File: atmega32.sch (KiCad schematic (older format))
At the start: 38 parts, among them J1 USB_B_Micro, J2 20021111-00016T4LF, SW1 SW_MEC_5E, U1 ATmega328P-AU, U2 FT232RL, Y1 Crystal

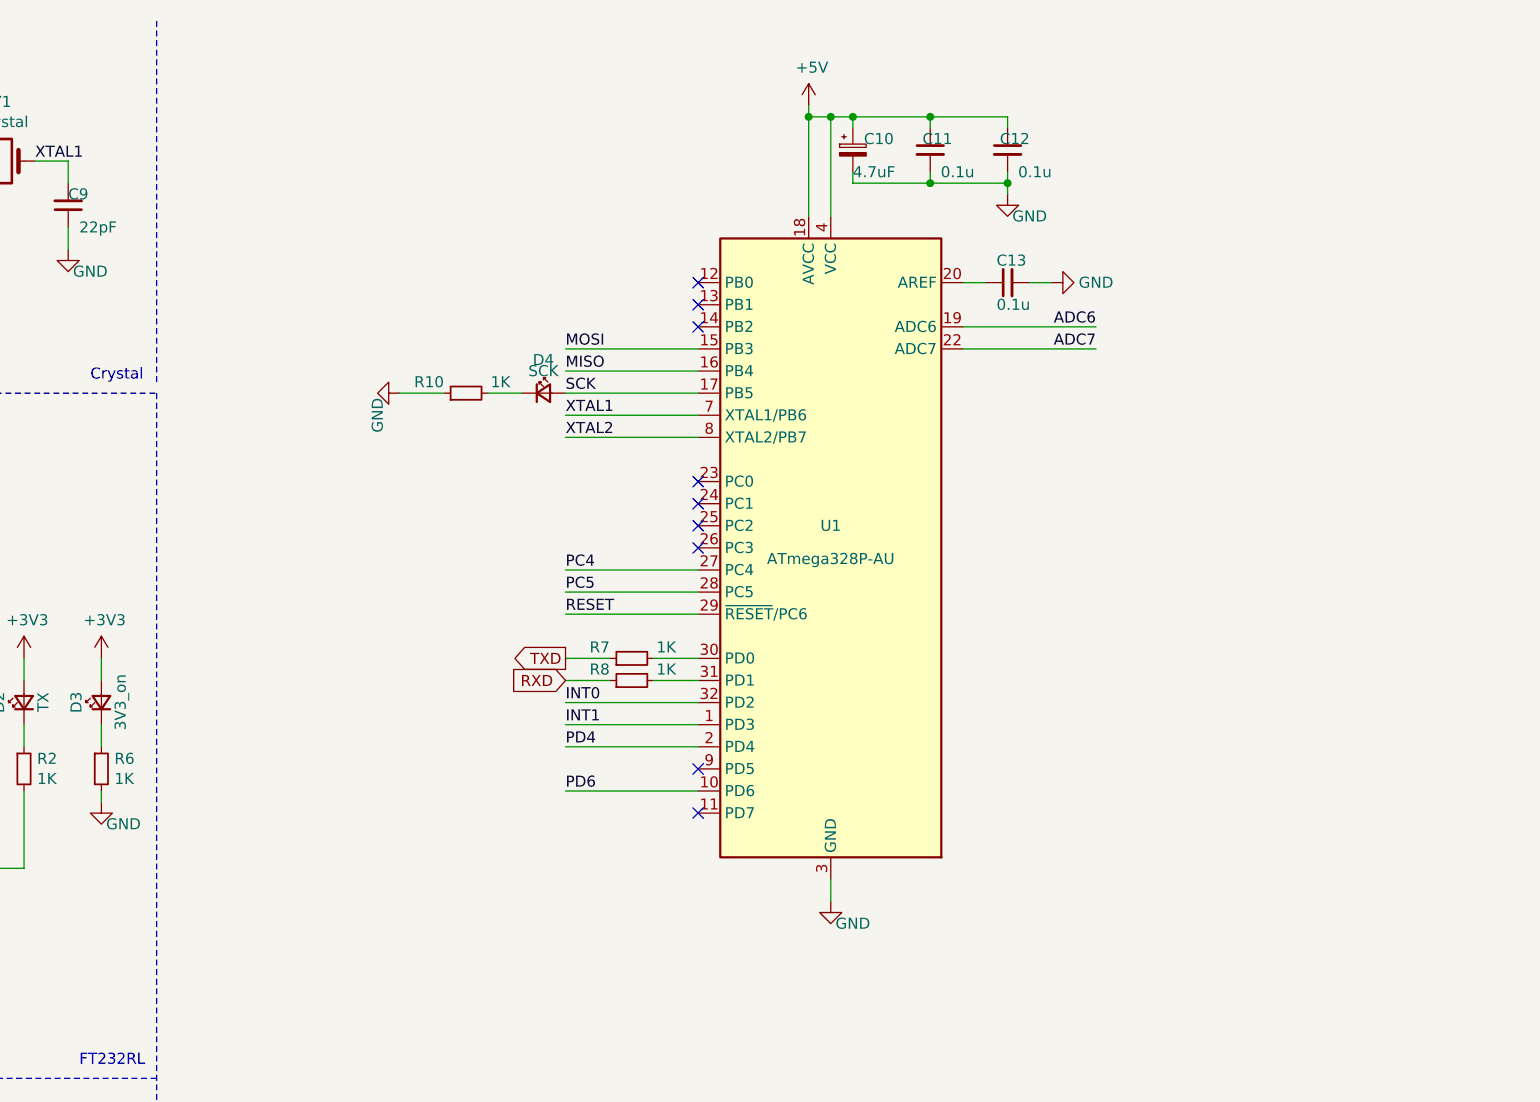
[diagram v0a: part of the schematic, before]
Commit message: orderd
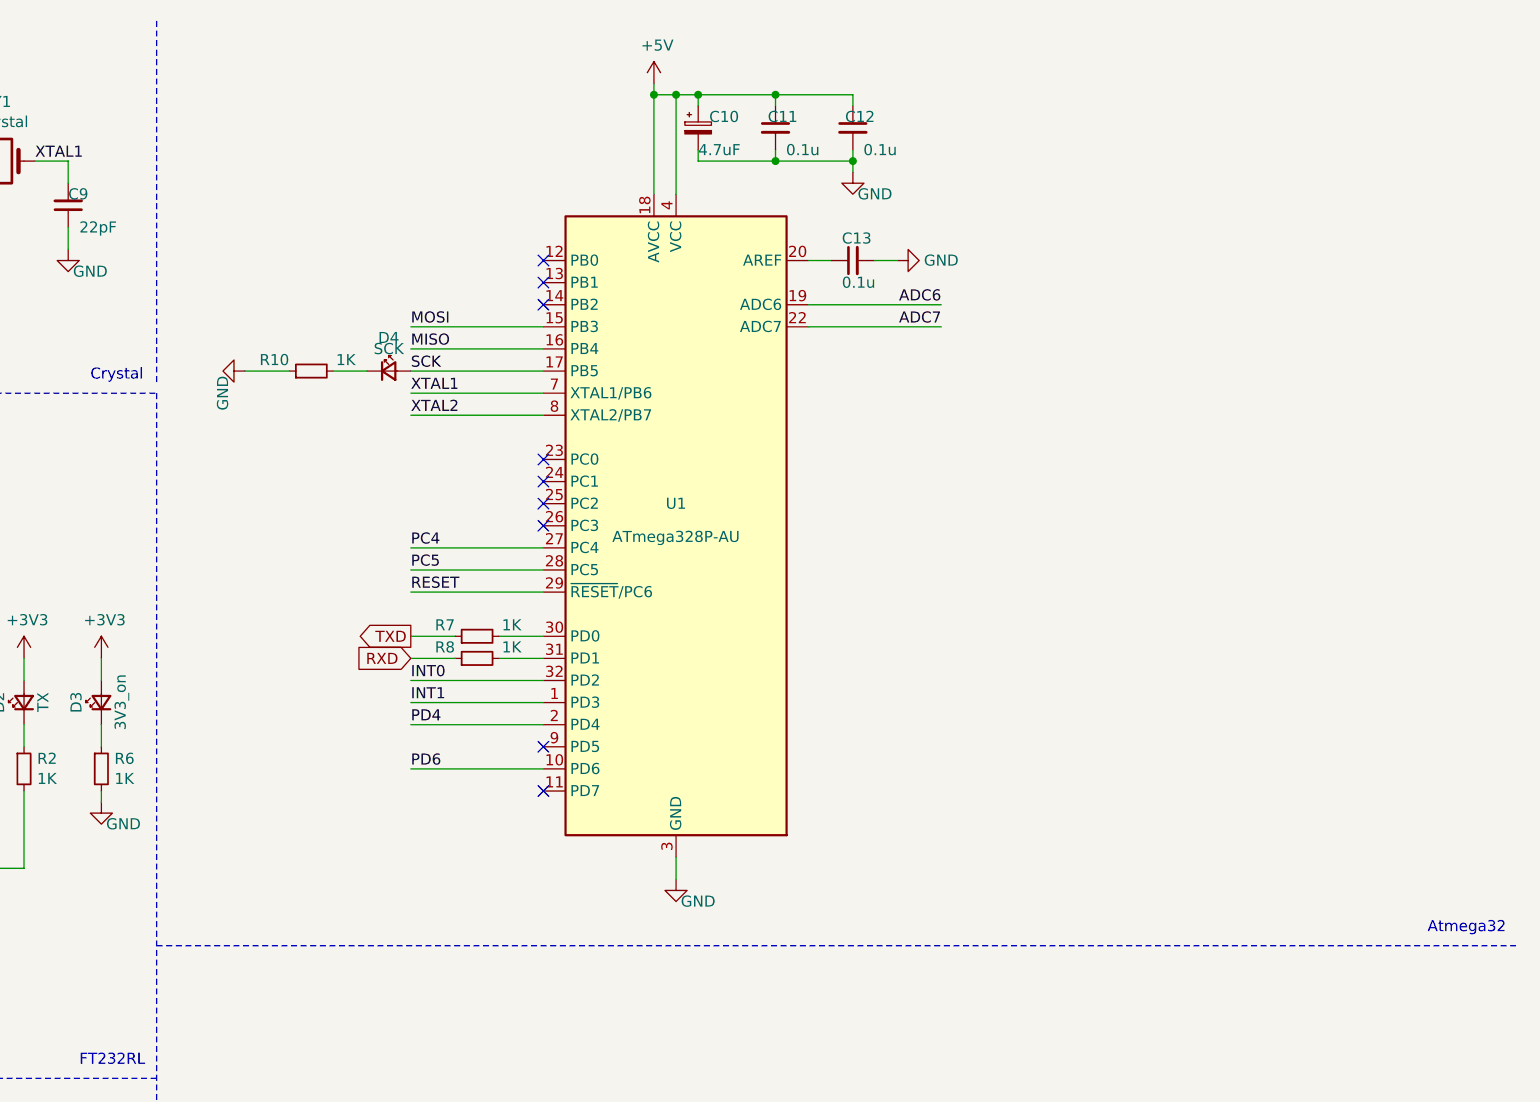
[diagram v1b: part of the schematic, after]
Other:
- note added: "Atmega32"
- moved on the sheet: C10, C11, C12, C13, D4, R10, R7, R8, U1
